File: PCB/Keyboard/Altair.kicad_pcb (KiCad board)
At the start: 2 copper layers, 134.8 x 110.6 mm, 70 parts, among them J1 Conn_01x02_Socket, J10 Jumper, J11 Jumper, J12 Jumper, J13 Jumper, J14 Jumper, J7 Jumper, J8 Jumper, J9 Jumper, SW1 SW_Push, SW10 SW_Push, SW11 SW_Push, SW12 SW_Push, SW13 SW_Push, SW14 SW_Push, SW15 SW_Push, SW16 SW_Push, SW17 SW_Push, SW18 SW_Push, SW19 SW_Push, SW2 SW_Push, SW20 SW_Push, SW21 SW_Push, SW22 SW_Push, SW23 SW_Push, SW24 SW_Push, SW25 SW_Push, SW26 SW_Push, SW27 SW_Push, SW28 SW_Push, SW3 SW_Push, SW4 SW_Push, SW5 SW_Push, SW6 SW_Push, SW7 SW_Push, SW8 SW_Push, SW9 SW_Push, SW97 SW_Nidec_CAS-120A1, SW98 RotaryEncoder_Switch, SW99 SW_Push, U1 SuperMini nRF52840

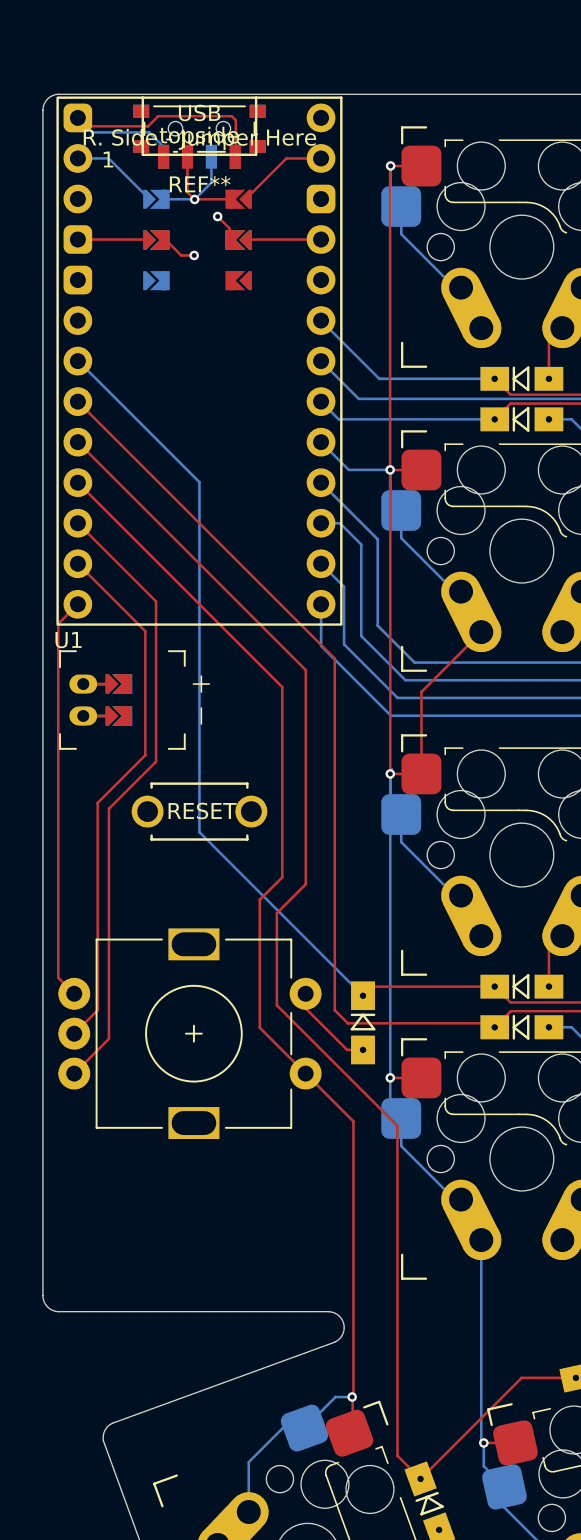
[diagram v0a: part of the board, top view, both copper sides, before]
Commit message: done & clean
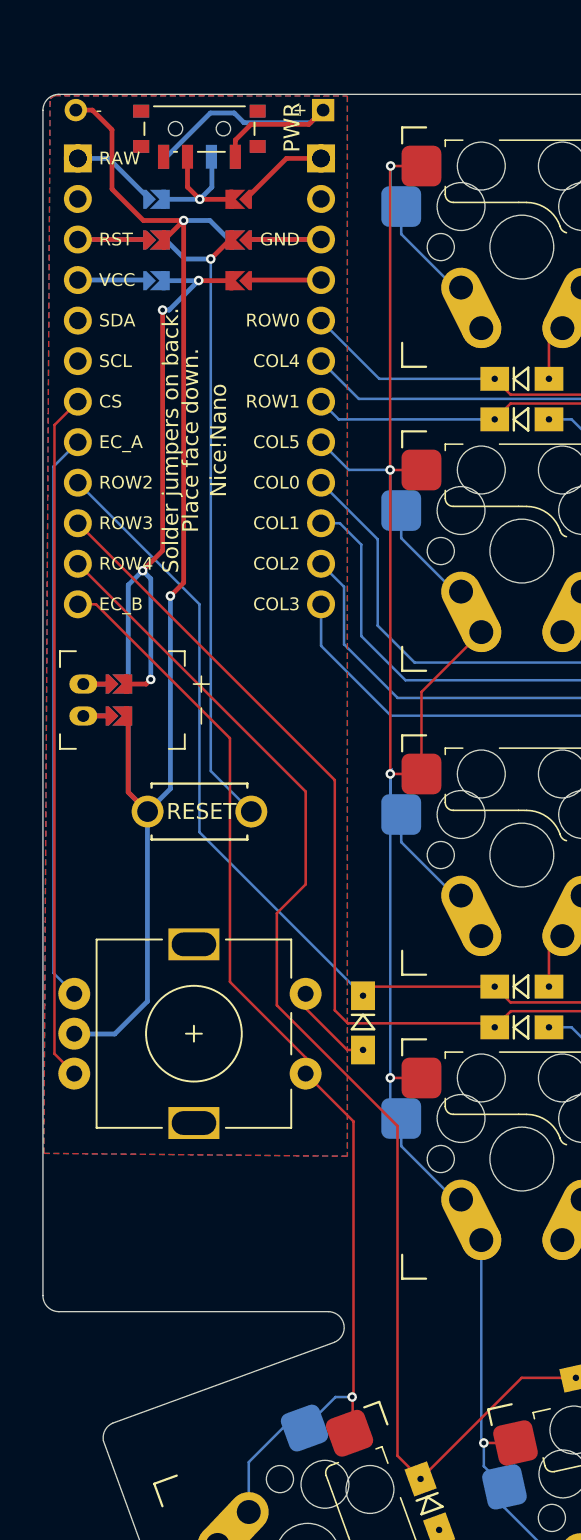
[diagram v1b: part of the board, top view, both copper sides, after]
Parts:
- removed U1: SuperMini nRF52840, PCM_marbastlib-xp-promicroish:SuperMini_nRF52840_AH_Reversible
- added ?: , lib:niceview_headers, B.Cu at (97.9, 40.2)
- added MCU1: , ProMicro, B.Cu at (97.9, 57.2)
- PWR: renamed from SW97; moved to F.Cu
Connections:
- J1 pad 1: unconnected-(J1-Pin_1-Pad1) -> GND
- J1 pad 2: unconnected-(J1-Pin_2-Pad2) -> GND
- J10 pad 1: (no net) -> RST_GND
- J10 pad 2: (no net) -> GND
- J11 pad 1: unconnected-(U1-BAT+-Pad13) -> RAW_P1
- J11 pad 2: (no net) -> RAW
- J12 pad 1: Net-(U1-RST) -> RST_GND
- J12 pad 2: Net-(U1-RST) -> RST
- J13 pad 1: (no net) -> VCC_GND
- J13 pad 2: (no net) -> VCC
- J14 pad 1: unconnected-(U1-GND-Pad3) -> GND_RST
- J14 pad 2: unconnected-(U1-GND-Pad3) -> GND
- J7 pad 1: unconnected-(U1-BAT+-Pad13) -> P1_RAW
- J7 pad 2: unconnected-(U1-BAT+-Pad13) -> RAW
- J8 pad 1: (no net) -> GND_RST
- J8 pad 2: (no net) -> RST
- J9 pad 1: (no net) -> GND_VCC
- J9 pad 2: (no net) -> VCC
- PWR pad 1: unconnected-(SW97-C-Pad1) -> switch_from
- PWR pad 2: unconnected-(SW97-B-Pad2) -> RAW
- SW98 pad C: EC_C -> GND
- SW99 pad 1: Net-(U1-RST) -> RST
- SW99 pad 2: unconnected-(U1-GND-Pad3) -> GND
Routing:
- net GND: track 20.0 -> 85.2 mm, vias 0 -> 2
- net RST: track 0.00 -> 41.0 mm, vias 0 -> 1
- net VCC: track 0.00 -> 39.9 mm, vias 0 -> 4
- net EC_C: track 33.0 -> 0.00 mm
- net unconnected-(U1-BAT+-Pad13): track 21.3 -> 0.00 mm, vias 1 -> 0
- net switch_from: track 0.00 -> 19.0 mm
- net EC_A: track 25.3 -> 35.7 mm
- net RST_GND: track 0.00 -> 9.48 mm
- net RAW: track 0.00 -> 9.16 mm, vias 0 -> 1
- net GND_RST: track 0.00 -> 9.01 mm
- net COL6: track 79.3 -> 71.2 mm
- net ROW2: track 159.2 -> 151.6 mm
- net ROW3: track 158.0 -> 150.3 mm
- net ROW4: track 131.9 -> 124.3 mm
- net Net-(U1-RST): track 6.84 -> 0.00 mm, vias 1 -> 0
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- added copper zone on B.Cu, net GND
- added copper zone on F.Cu, net GND
